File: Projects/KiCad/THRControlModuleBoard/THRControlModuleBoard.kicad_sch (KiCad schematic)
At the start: 25 parts, among them J1 Screw_Terminal_01x02, J5 Conn_02x03_Odd_Even, J6 Conn_02x03_Odd_Even, U1 MAX31856MUD+T

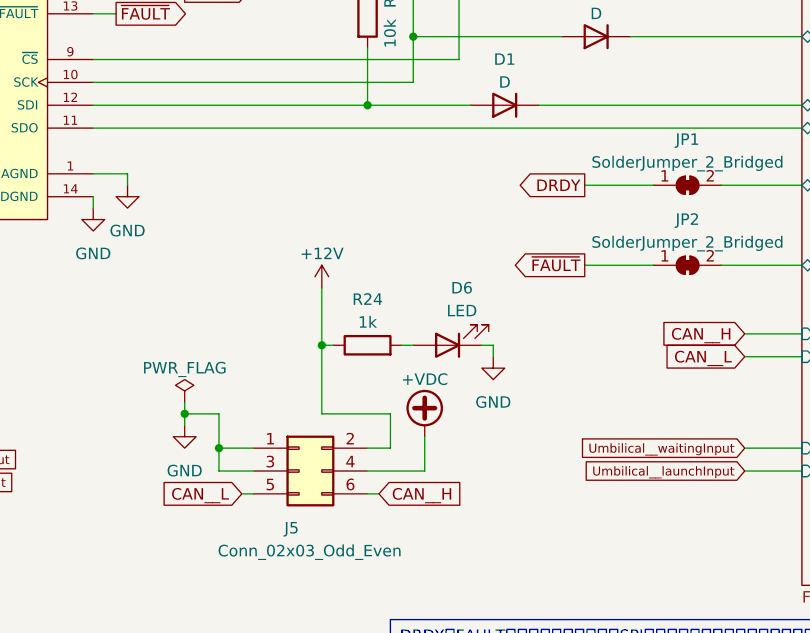
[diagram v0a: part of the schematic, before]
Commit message: 長時間の動作を確認した。
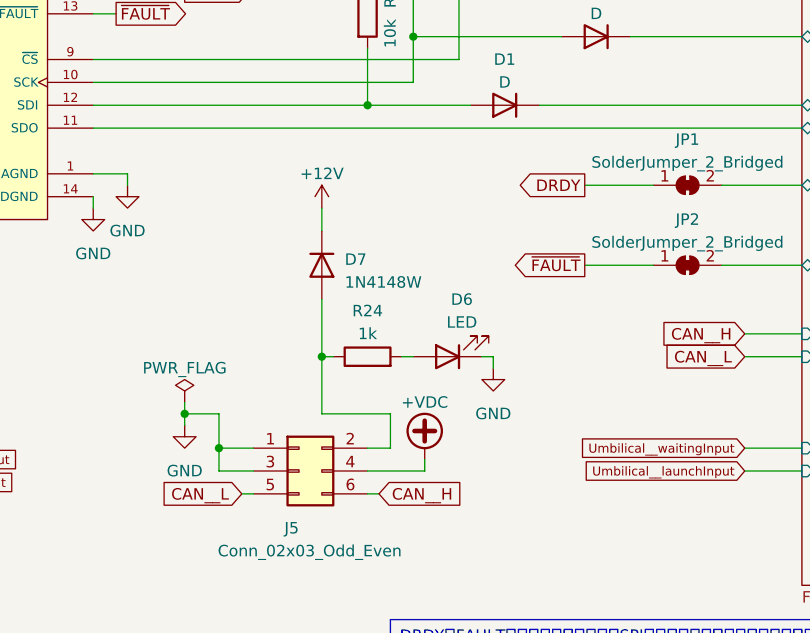
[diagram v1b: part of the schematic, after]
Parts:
- added D7: 1N4148W, Diode_SMD:D_SOD-123, symbol Diode:1N4148W
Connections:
- net +12V: now also D7.1 (K); no longer J5.2 (Pin_2), R24.1
- new net: D7.2 (A), J5.2 (Pin_2), R24.1
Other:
- moved on the sheet: D6, R24
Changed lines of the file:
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@@
   (junction (at 209.55 59.69) (diameter 0) (color 0 0 0 0)
   )
-  (junction (at 199.39 93.98) (diameter 0) (color 0 0 0 0)
-  )
   (junction (at 214.63 52.07) (diameter 0) (color 0 0 0 0)
   )
@@
   (junction (at 144.78 111.76) (diameter 0) (color 0 0 0 0)
   )
+  (junction (at 199.39 95.25) (diameter 0) (color 0 0 0 0)
+  )
   (junction (at 123.19 106.68) (diameter 0) (color 0 0 0 0)
   )
@@
   (junction (at 184.15 101.6) (diameter 0) (color 0 0 0 0)
   )
-  (wire (pts (xy 210.82 104.14) (xy 210.82 107.95))
+  (wire (pts (xy 210.82 106.68) (xy 210.82 107.95))
     (stroke (width 0) (type default))
   )
@@
     (stroke (width 0) (type default))
   )
-  (wire (pts (xy 217.17 93.98) (xy 218.44 93.98))
+  (wire (pts (xy 218.44 95.25) (xy 218.44 96.52))
+    (stroke (width 0) (type default))
+  )
+  (wire (pts (xy 199.39 88.9) (xy 199.39 95.25))
     (stroke (width 0) (type default))
   )
@@
     (stroke (width 0) (type default))
   )
-  (wire (pts (xy 200.66 93.98) (xy 199.39 93.98))
-    (stroke (width 0) (type default))
-  )
   (wire (pts (xy 204.47 67.31) (xy 215.9 67.31))
     (stroke (width 0) (type default))
@@
     (stroke (width 0) (type default))
   )
-  (wire (pts (xy 199.39 87.63) (xy 199.39 93.98))
-    (stroke (width 0) (type default))
-  )
   (wire (pts (xy 199.39 101.6) (xy 207.01 101.6))
     (stroke (width 0) (type default))
@@
     (stroke (width 0) (type default))
   )
+  (wire (pts (xy 199.39 78.74) (xy 199.39 81.28))
+    (stroke (width 0) (type default))
+  )
   (wire (pts (xy 146.05 111.76) (xy 144.78 111.76))
     (stroke (width 0) (type default))
@@
     (stroke (width 0) (type default))
   )
-  (wire (pts (xy 218.44 93.98) (xy 218.44 95.25))
-    (stroke (width 0) (type default))
-  )
   (wire (pts (xy 175.26 27.94) (xy 175.26 34.29))
     (stroke (width 0) (type default))
@@
     (stroke (width 0) (type default))
   )
+  (wire (pts (xy 199.39 95.25) (xy 200.66 95.25))
+    (stroke (width 0) (type default))
+  )
   (wire (pts (xy 246.38 105.41) (xy 252.73 105.41))
     (stroke (width 0) (type default))
   )
+  (wire (pts (xy 218.44 95.25) (xy 217.17 95.25))
+    (stroke (width 0) (type default))
+  )
   (wire (pts (xy 97.79 54.61) (xy 106.68 54.61))
     (stroke (width 0) (type default))
   )
-  (wire (pts (xy 199.39 93.98) (xy 199.39 101.6))
-    (stroke (width 0) (type default))
-  )
   (wire (pts (xy 187.96 107.95) (xy 187.96 105.41))
     (stroke (width 0) (type default))
@@
     (stroke (width 0) (type default))
   )
+  (wire (pts (xy 199.39 95.25) (xy 199.39 101.6))
+    (stroke (width 0) (type default))
+  )
   (wire (pts (xy 175.26 34.29) (xy 175.26 46.99))
     (stroke (width 0) (type default))
@@
     (stroke (width 0) (type default))
   )
-  (wire (pts (xy 208.28 93.98) (xy 209.55 93.98))
+  (wire (pts (xy 208.28 95.25) (xy 209.55 95.25))
     (stroke (width 0) (type default))
   )
@@
     )
   )
-  (symbol (lib_id "power:+12V") (at 199.39 87.63 0) (unit 1)
-    (in_bom yes) (on_board yes) (dnp no) (fields_autoplaced)
-    (property "Reference" "#PWR040" (at 199.39 91.44 0)
-      (effects (font (size 1.27 1.27)) hide)
-    )
-    (property "Value" "+12V" (at 199.39 83.82 0)
-      (effects (font (size 1.27 1.27)))
-    )
-    (property "Footprint" "" (at 199.39 87.63 0)
-      (effects (font (size 1.27 1.27)) hide)
-    )
-    (property "Datasheet" "" (at 199.39 87.63 0)
+  (symbol (lib_id "power:+12V") (at 199.39 78.74 0) (unit 1)
+    (in_bom yes) (on_board yes) (dnp no) (fields_autoplaced)
+    (property "Reference" "#PWR040" (at 199.39 82.55 0)
+      (effects (font (size 1.27 1.27)) hide)
+    )
+    (property "Value" "+12V" (at 199.39 74.93 0)
+      (effects (font (size 1.27 1.27)))
+    )
+    (property "Footprint" "" (at 199.39 78.74 0)
+      (effects (font (size 1.27 1.27)) hide)
+    )
+    (property "Datasheet" "" (at 199.39 78.74 0)
       (effects (font (size 1.27 1.27)) hide)
     )
@@
     )
   )
-  (symbol (lib_id "Device:LED") (at 213.36 93.98 180) (unit 1)
-    (in_bom yes) (on_board yes) (dnp no) (fields_autoplaced)
-    (property "Reference" "D6" (at 214.9475 87.63 0)
-      (effects (font (size 1.27 1.27)))
-    )
-    (property "Value" "LED" (at 214.9475 90.17 0)
-      (effects (font (size 1.27 1.27)))
-    )
-    (property "Footprint" "LED_SMD:LED_0603_1608Metric_Pad1.05x0.95mm_HandSolder" (at 213.36 93.98 0)
-      (effects (font (size 1.27 1.27)) hide)
-    )
-    (property "Datasheet" "~" (at 213.36 93.98 0)
+  (symbol (lib_id "Device:LED") (at 213.36 95.25 180) (unit 1)
+    (in_bom yes) (on_board yes) (dnp no) (fields_autoplaced)
+    (property "Reference" "D6" (at 214.9475 88.9 0)
+      (effects (font (size 1.27 1.27)))
+    )
+    (property "Value" "LED" (at 214.9475 91.44 0)
+      (effects (font (size 1.27 1.27)))
+    )
+    (property "Footprint" "LED_SMD:LED_0603_1608Metric_Pad1.05x0.95mm_HandSolder" (at 213.36 95.25 0)
+      (effects (font (size 1.27 1.27)) hide)
+    )
+    (property "Datasheet" "~" (at 213.36 95.25 0)
       (effects (font (size 1.27 1.27)) hide)
     )
@@
     )
   )
-  (symbol (lib_id "power:+VDC") (at 210.82 104.14 0) (unit 1)
-    (in_bom yes) (on_board yes) (dnp no) (fields_autoplaced)
-    (property "Reference" "#PWR013" (at 210.82 106.68 0)
-      (effects (font (size 1.27 1.27)) hide)
-    )
-    (property "Value" "+VDC" (at 210.82 97.79 0)
-      (effects (font (size 1.27 1.27)))
-    )
-    (property "Footprint" "" (at 210.82 104.14 0)
-      (effects (font (size 1.27 1.27)) hide)
-    )
-    (property "Datasheet" "" (at 210.82 104.14 0)
+  (symbol (lib_id "power:+VDC") (at 210.82 106.68 0) (unit 1)
+    (in_bom yes) (on_board yes) (dnp no) (fields_autoplaced)
+    (property "Reference" "#PWR013" (at 210.82 109.22 0)
+      (effects (font (size 1.27 1.27)) hide)
+    )
+    (property "Value" "+VDC" (at 210.82 100.33 0)
+      (effects (font (size 1.27 1.27)))
+    )
+    (property "Footprint" "" (at 210.82 106.68 0)
+      (effects (font (size 1.27 1.27)) hide)
+    )
+    (property "Datasheet" "" (at 210.82 106.68 0)
       (effects (font (size 1.27 1.27)) hide)
     )
@@
     )
   )
-  (symbol (lib_id "power:GND") (at 218.44 95.25 0) (unit 1)
-    (in_bom yes) (on_board yes) (dnp no) (fields_autoplaced)
-    (property "Reference" "#PWR053" (at 218.44 101.6 0)
-      (effects (font (size 1.27 1.27)) hide)
-    )
-    (property "Value" "GND" (at 218.44 100.33 0)
-      (effects (font (size 1.27 1.27)))
-    )
-    (property "Footprint" "" (at 218.44 95.25 0)
-      (effects (font (size 1.27 1.27)) hide)
-    )
-    (property "Datasheet" "" (at 218.44 95.25 0)
+  (symbol (lib_id "power:GND") (at 218.44 96.52 0) (unit 1)
+    (in_bom yes) (on_board yes) (dnp no) (fields_autoplaced)
+    (property "Reference" "#PWR053" (at 218.44 102.87 0)
+      (effects (font (size 1.27 1.27)) hide)
+    )
+    (property "Value" "GND" (at 218.44 101.6 0)
+      (effects (font (size 1.27 1.27)))
+    )
+    (property "Footprint" "" (at 218.44 96.52 0)
+      (effects (font (size 1.27 1.27)) hide)
+    )
+    (property "Datasheet" "" (at 218.44 96.52 0)
       (effects (font (size 1.27 1.27)) hide)
     )
@@
         (path "/79fd2516-dad6-414c-bb46-91ee9bfb5006"
           (reference "R3") (unit 1)
+        )
+      )
+    )
+  )
+  (symbol (lib_id "Diode:1N4148W") (at 199.39 85.09 270) (unit 1)
+    (in_bom yes) (on_board yes) (dnp no) (fields_autoplaced)
+    (property "Reference" "D7" (at 201.93 84.455 90)
+      (effects (font (size 1.27 1.27)) (justify left))
+    )
+    (property "Value" "1N4148W" (at 201.93 86.995 90)
+      (effects (font (size 1.27 1.27)) (justify left))
+    )
+    (property "Footprint" "Diode_SMD:D_SOD-123" (at 194.945 85.09 0)
+      (effects (font (size 1.27 1.27)) hide)
+    )
+    (property "Datasheet" "https://www.vishay.com/docs/85748/1n4148w.pdf" (at 199.39 85.09 0)
+      (effects (font (size 1.27 1.27)) hide)
+    )
+    (property "Sim.Device" "D" (at 199.39 85.09 0)
+      (effects (font (size 1.27 1.27)) hide)
+    )
+    (property "Sim.Pins" "1=K 2=A" (at 199.39 85.09 0)
+      (effects (font (size 1.27 1.27)) hide)
+    )
+    (pin "1")
+    (pin "2")
+    (instances
+      (project "THRControlModuleBoard"
+        (path "/79fd2516-dad6-414c-bb46-91ee9bfb5006"
+          (reference "D7") (unit 1)
         )
       )
@@
     )
   )
-  (symbol (lib_id "Device:R") (at 204.47 93.98 90) (unit 1)
-    (in_bom yes) (on_board yes) (dnp no) (fields_autoplaced)
-    (property "Reference" "R24" (at 204.47 88.9 90)
-      (effects (font (size 1.27 1.27)))
-    )
-    (property "Value" "1k" (at 204.47 91.44 90)
-      (effects (font (size 1.27 1.27)))
-    )
-    (property "Footprint" "Resistor_SMD:R_0603_1608Metric_Pad0.98x0.95mm_HandSolder" (at 204.47 95.758 90)
-      (effects (font (size 1.27 1.27)) hide)
-    )
-    (property "Datasheet" "~" (at 204.47 93.98 0)
-      (effects (font (size 1.27 1.27)) hide)
-    )
+  (symbol (lib_id "Device:R") (at 204.47 95.25 90) (unit 1)
+    (in_bom yes) (on_board yes) (dnp no) (fields_autoplaced)
+    (property "Reference" "R24" (at 204.47 90.17 90)
+      (effects (font (size 1.27 1.27)))
+    )
+    (property "Value" "1k" (at 204.47 92.71 90)
+      (effects (font (size 1.27 1.27)))
+    )
+    (property "Footprint" "Resistor_SMD:R_0603_1608Metric_Pad0.98x0.95mm_HandSolder" (at 204.47 97.028 90)
+      (effects (font (size 1.27 1.27)) hide)
+    )
+    (property "Datasheet" "~" (at 204.47 95.25 0)
+      (effects (font (size 1.27 1.27)) hide)
+    )
